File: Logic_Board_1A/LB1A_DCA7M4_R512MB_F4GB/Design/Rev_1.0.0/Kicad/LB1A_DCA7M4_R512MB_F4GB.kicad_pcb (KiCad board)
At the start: 6 copper layers, 50 x 50 mm, 143 parts, among them U1 STM32MP157CAC3, U2 AS4C256M16D3LC-12BCN, U3 S40FC004C1B2C00000, U4 STPMIC1BPQR, U5 DF40C-70DP-0.4V(51), U6 DF40C-70DP-0.4V(51), U7 DF40C-70DP-0.4V(51), X1 32.768kHz, X2 24MHz

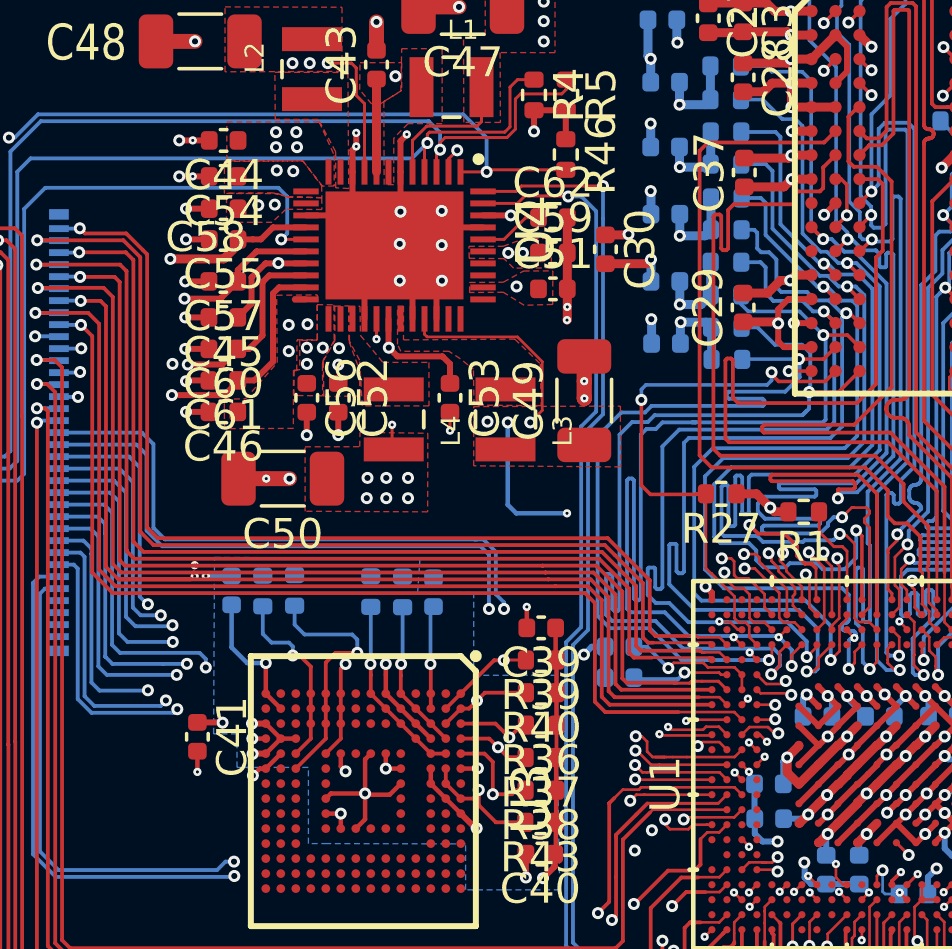
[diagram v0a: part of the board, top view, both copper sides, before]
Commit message: NO DRC & UNCONNECTED
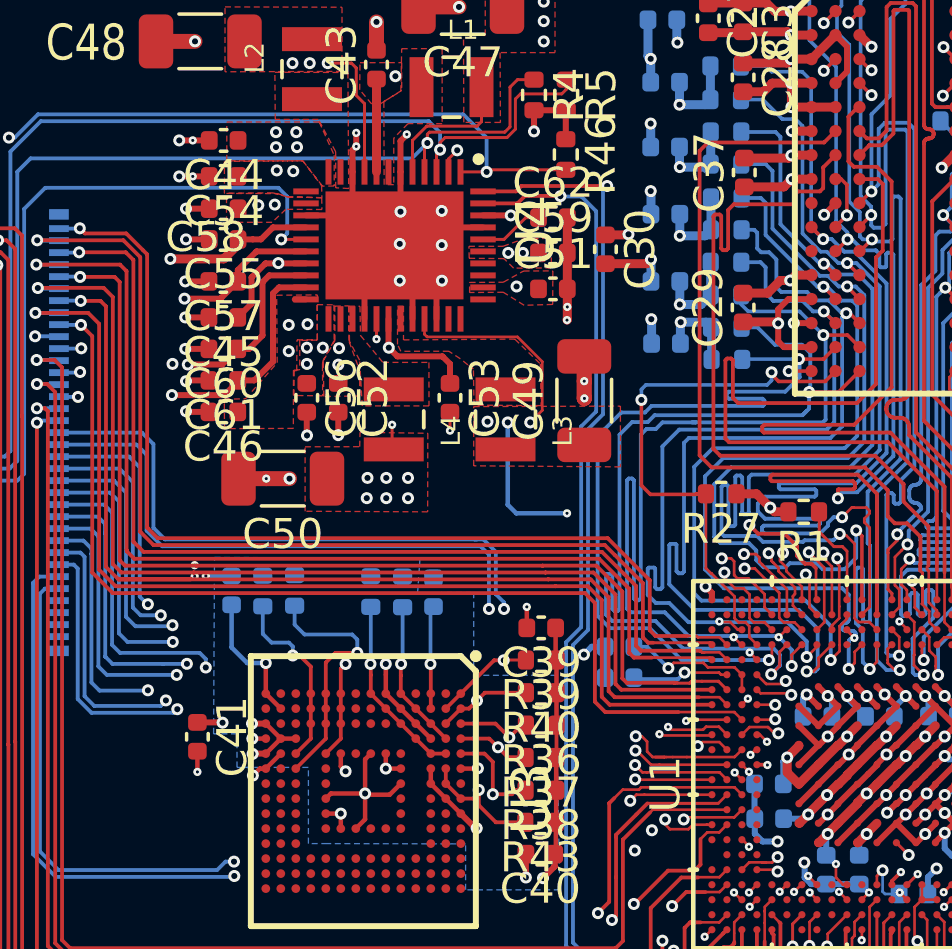
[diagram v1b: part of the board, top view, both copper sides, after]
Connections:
- U6 pad 1: GND -> PMIC_VOUT4_3V3
- U6 pad 27: PMIC_VOUT4_3V3 -> GND
- U6 pad 29: PMIC_VOUT4_3V3 -> GND
- U6 pad 3: GND -> PMIC_VOUT4_3V3
- U6 pad 31: PMIC_VOUT4_3V3 -> GND
- U6 pad 33: PMIC_VOUT4_3V3 -> GND
- U6 pad 35: PMIC_VOUT4_3V3 -> GND
- U6 pad 5: GND -> PMIC_VOUT4_3V3
- U6 pad 7: GND -> PMIC_VOUT4_3V3
- U6 pad 9: GND -> PMIC_VOUT4_3V3
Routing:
- net PMIC_LDO1_1V8: track 30.8 -> 29.9 mm
- net PMIC_LDO2_2V9: track 32.5 -> 31.7 mm
- net PMIC_VOUT4_3V3: track 8.80 -> 9.32 mm
- added copper zone on Signal_Layer_2.Cu, net PMIC_VOUT4_3V3
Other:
- net class DDR_DiffPairs: clearance 0.1016 -> 0.0762
- net class Default: clearance 0.1016 -> 0.0762
- net class Gnd_Lines: clearance 0.1016 -> 0.0762
- rule trace_clearance: 0.1016 -> 0.0762

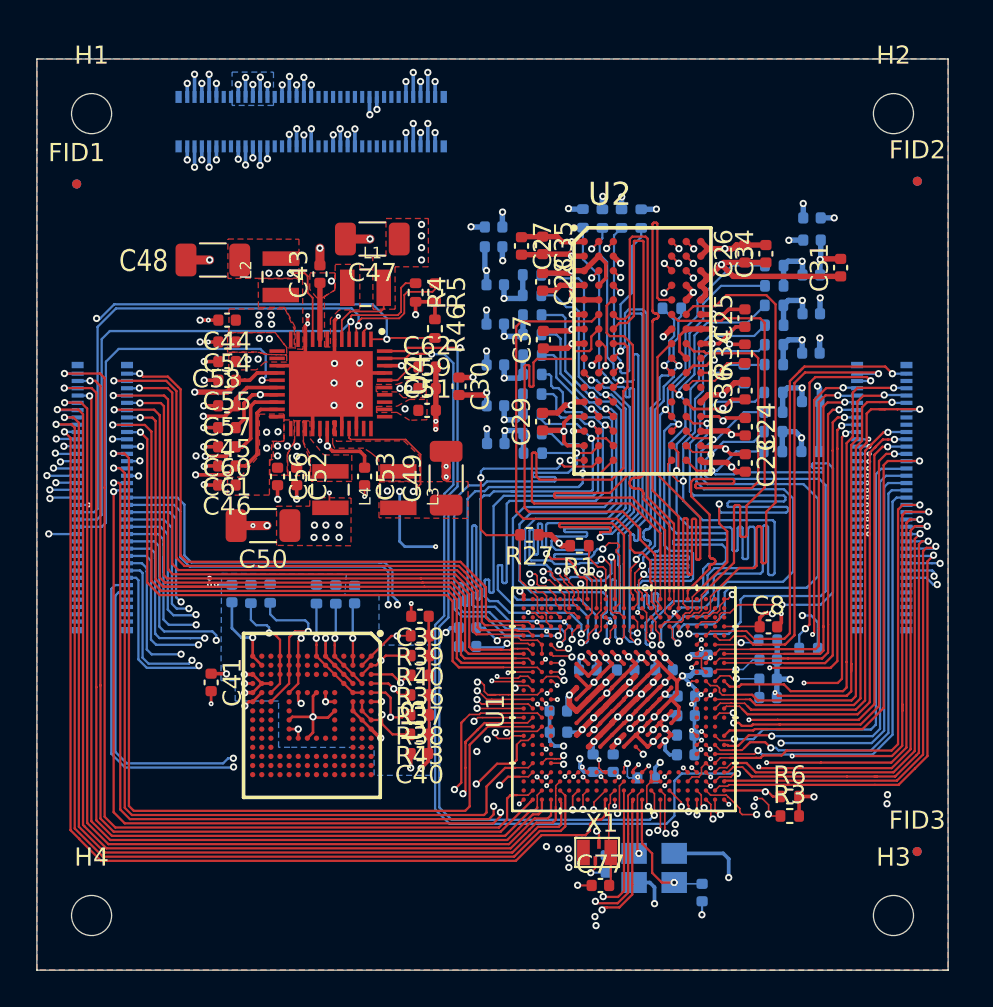
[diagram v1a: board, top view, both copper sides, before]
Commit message: more improvements
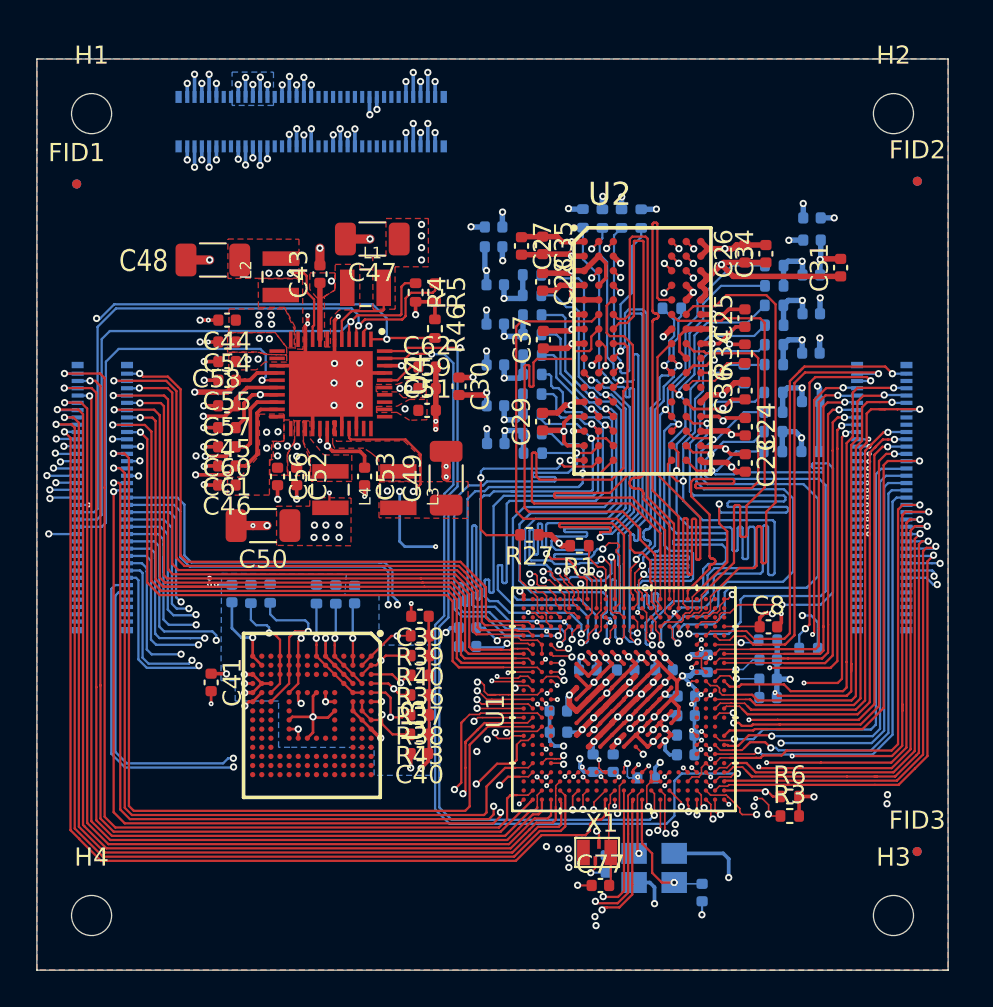
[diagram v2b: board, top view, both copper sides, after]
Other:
- net class DDR_DiffPairs: clearance 0.0762 -> 0.1016
- net class Default: clearance 0.0762 -> 0.1016
- net class Gnd_Lines: clearance 0.0762 -> 0.1016
- rule trace_clearance: 0.0762 -> 0.1016
